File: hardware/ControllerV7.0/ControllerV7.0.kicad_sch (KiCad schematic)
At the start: 9 parts, among them M1 Stepper_Motor_bipolar, M2 Stepper_Motor_bipolar, M3 Stepper_Motor_bipolar, M4 Stepper_Motor_bipolar, M5 Stepper_Motor_bipolar, M6 Stepper_Motor_bipolar

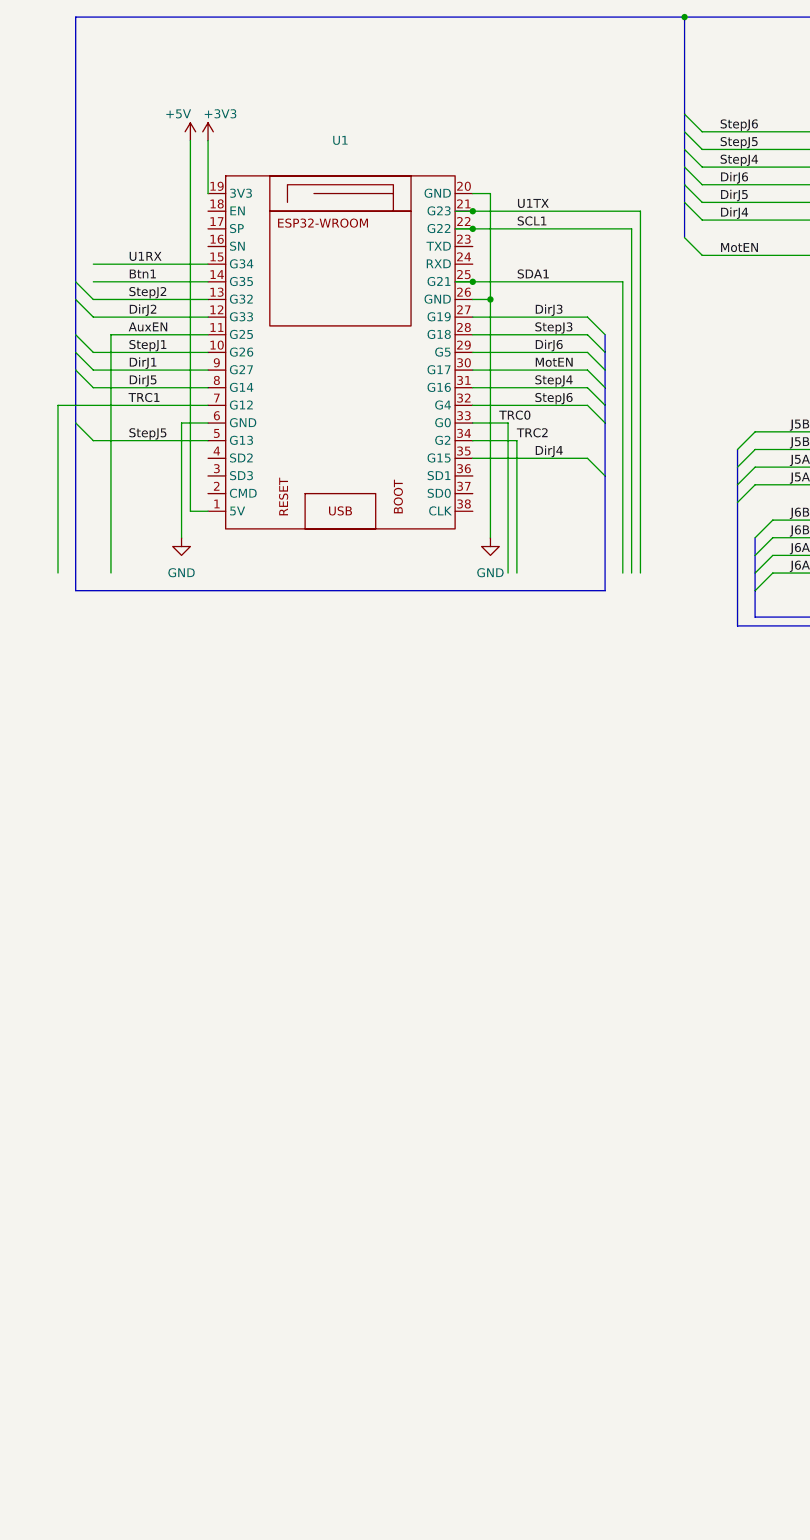
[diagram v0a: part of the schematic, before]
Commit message: Baseline before adding GCode and Planner
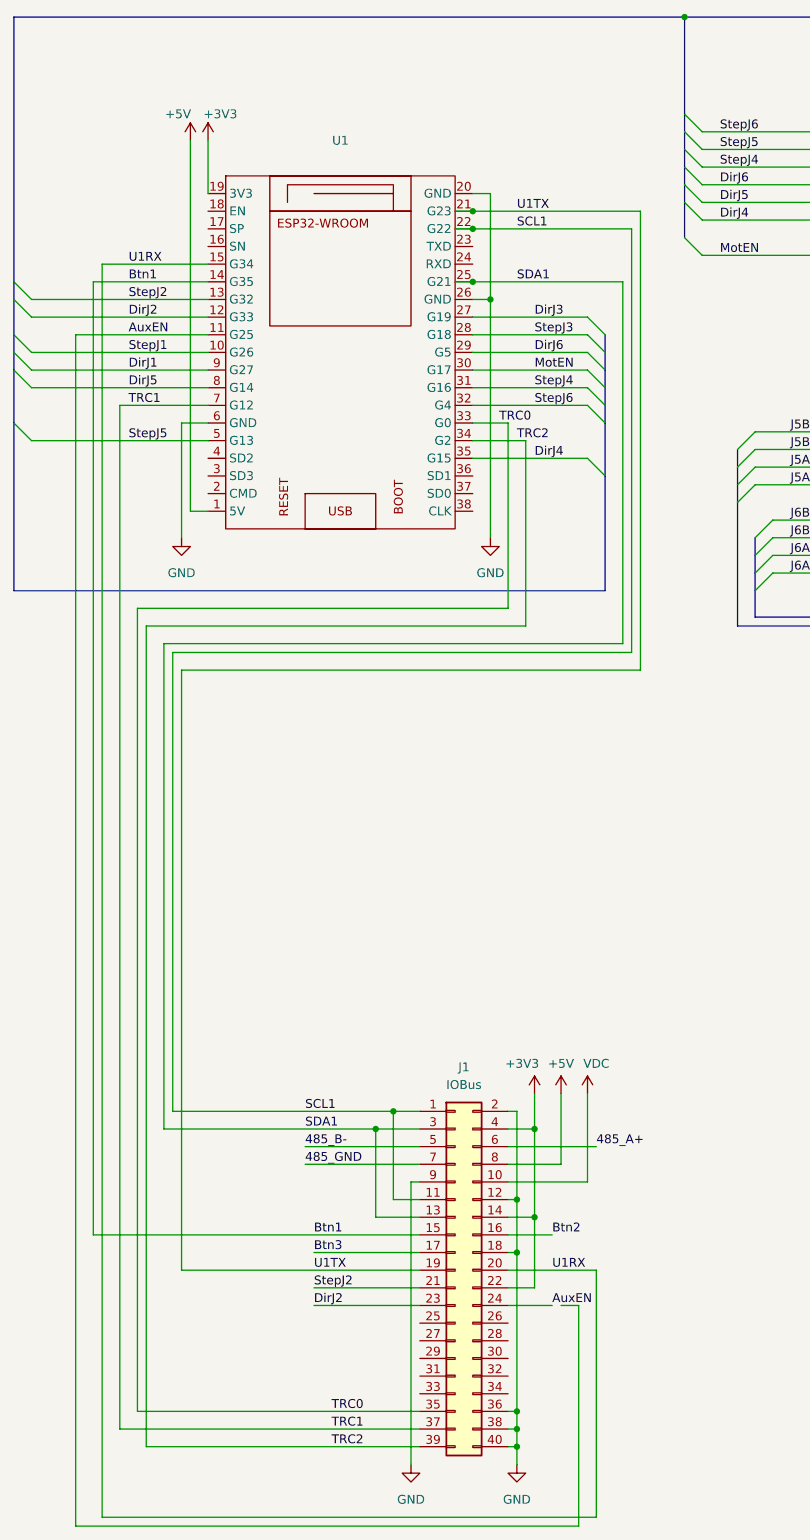
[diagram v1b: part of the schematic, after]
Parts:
- added J1: IOBus, symbol Connector_Generic:Conn_02x20_Odd_Even
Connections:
- net +3V3: now also J1.14 (Pin_14), J1.22 (Pin_22), J1.4 (Pin_4)
- net +5V: now also J1.8 (Pin_8)
- net AuxEN: now also J1.24 (Pin_24)
- net Btn1: now also J1.15 (Pin_15)
- net DirJ2: now also J1.23 (Pin_23)
- net GND: now also J1.12 (Pin_12), J1.18 (Pin_18), J1.2 (Pin_2), J1.36 (Pin_36), J1.38 (Pin_38), J1.40 (Pin_40), J1.9 (Pin_9)
- net SCL1: now also J1.1 (Pin_1), J1.11 (Pin_11)
- net SDA1: now also J1.13 (Pin_13), J1.3 (Pin_3)
- net StepJ2: now also J1.21 (Pin_21)
- net TRC0: now also J1.35 (Pin_35)
- net TRC1: now also J1.37 (Pin_37)
- net TRC2: now also J1.39 (Pin_39)
- net U1RX: now also J1.20 (Pin_20)
- net U1TX: now also J1.19 (Pin_19)
- net VDC: now also J1.10 (Pin_10)
- new net 485_A+: J1.6 (Pin_6)
- new net 485_B-: J1.5 (Pin_5)
- new net 485_GND: J1.7 (Pin_7)
- new net Btn2: J1.16 (Pin_16)
- new net Btn3: J1.17 (Pin_17)
